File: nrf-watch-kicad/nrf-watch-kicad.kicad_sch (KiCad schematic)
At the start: 78 parts, among them IC1 TLV840MAPL36DBVRQ1, IC2 XC9265C181MR-G, IC3 TPS61023DRLT, IC4 MAX30101EFD+T, M1 Vibrator DC Motor, Q1 DMP2045U-7, Q2 SS8050-G, U1 MAX1811ESA+, U2 DMC2400UV-7, U3 LIS2DS12TR, U4 MX25R6435FZNIL0, U5 u-blox ANNA-B402, U6 DRV2603RUNT, U7 XC9265A331MR-G, U8 TXB0104QRUTRQ1, U9 GC9A01

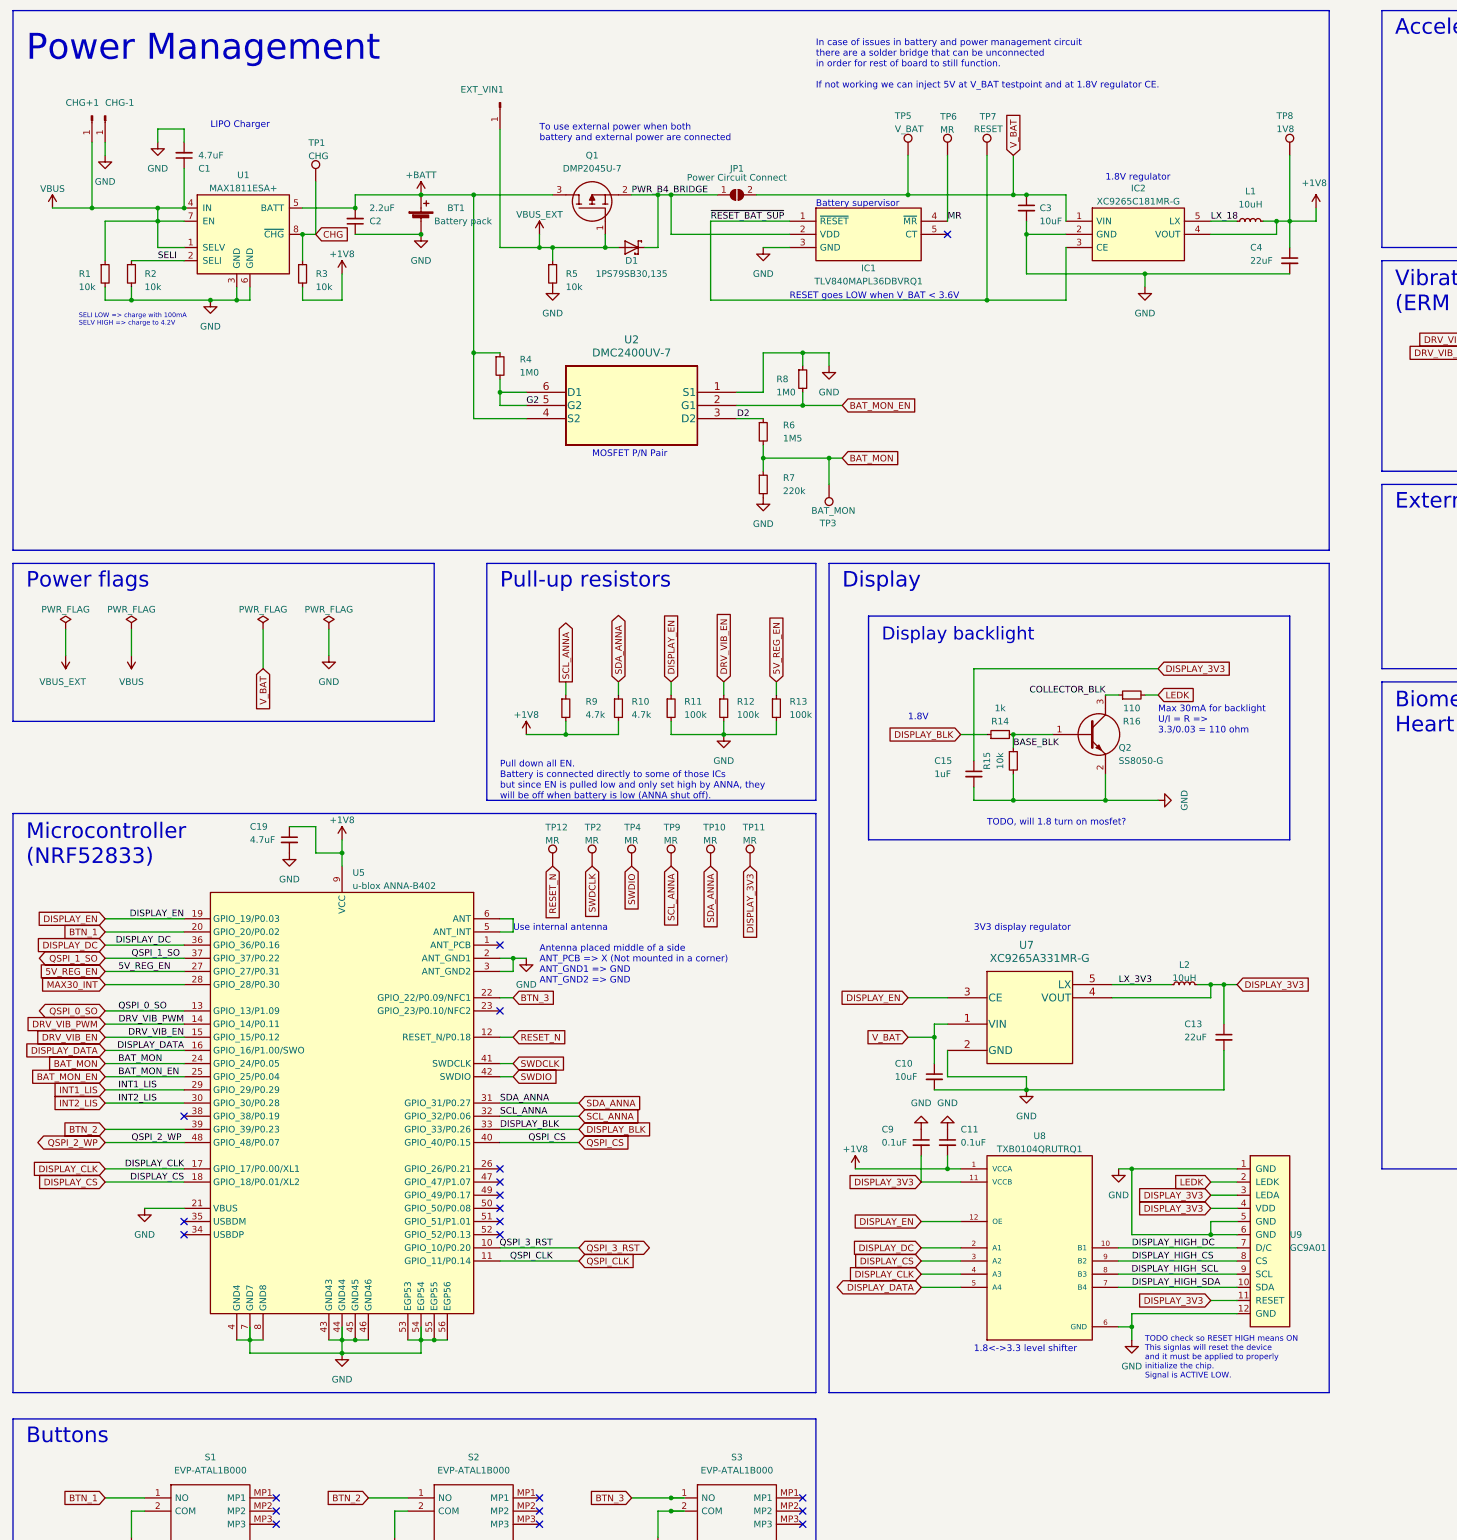
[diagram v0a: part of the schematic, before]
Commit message: Before moving bottom to top
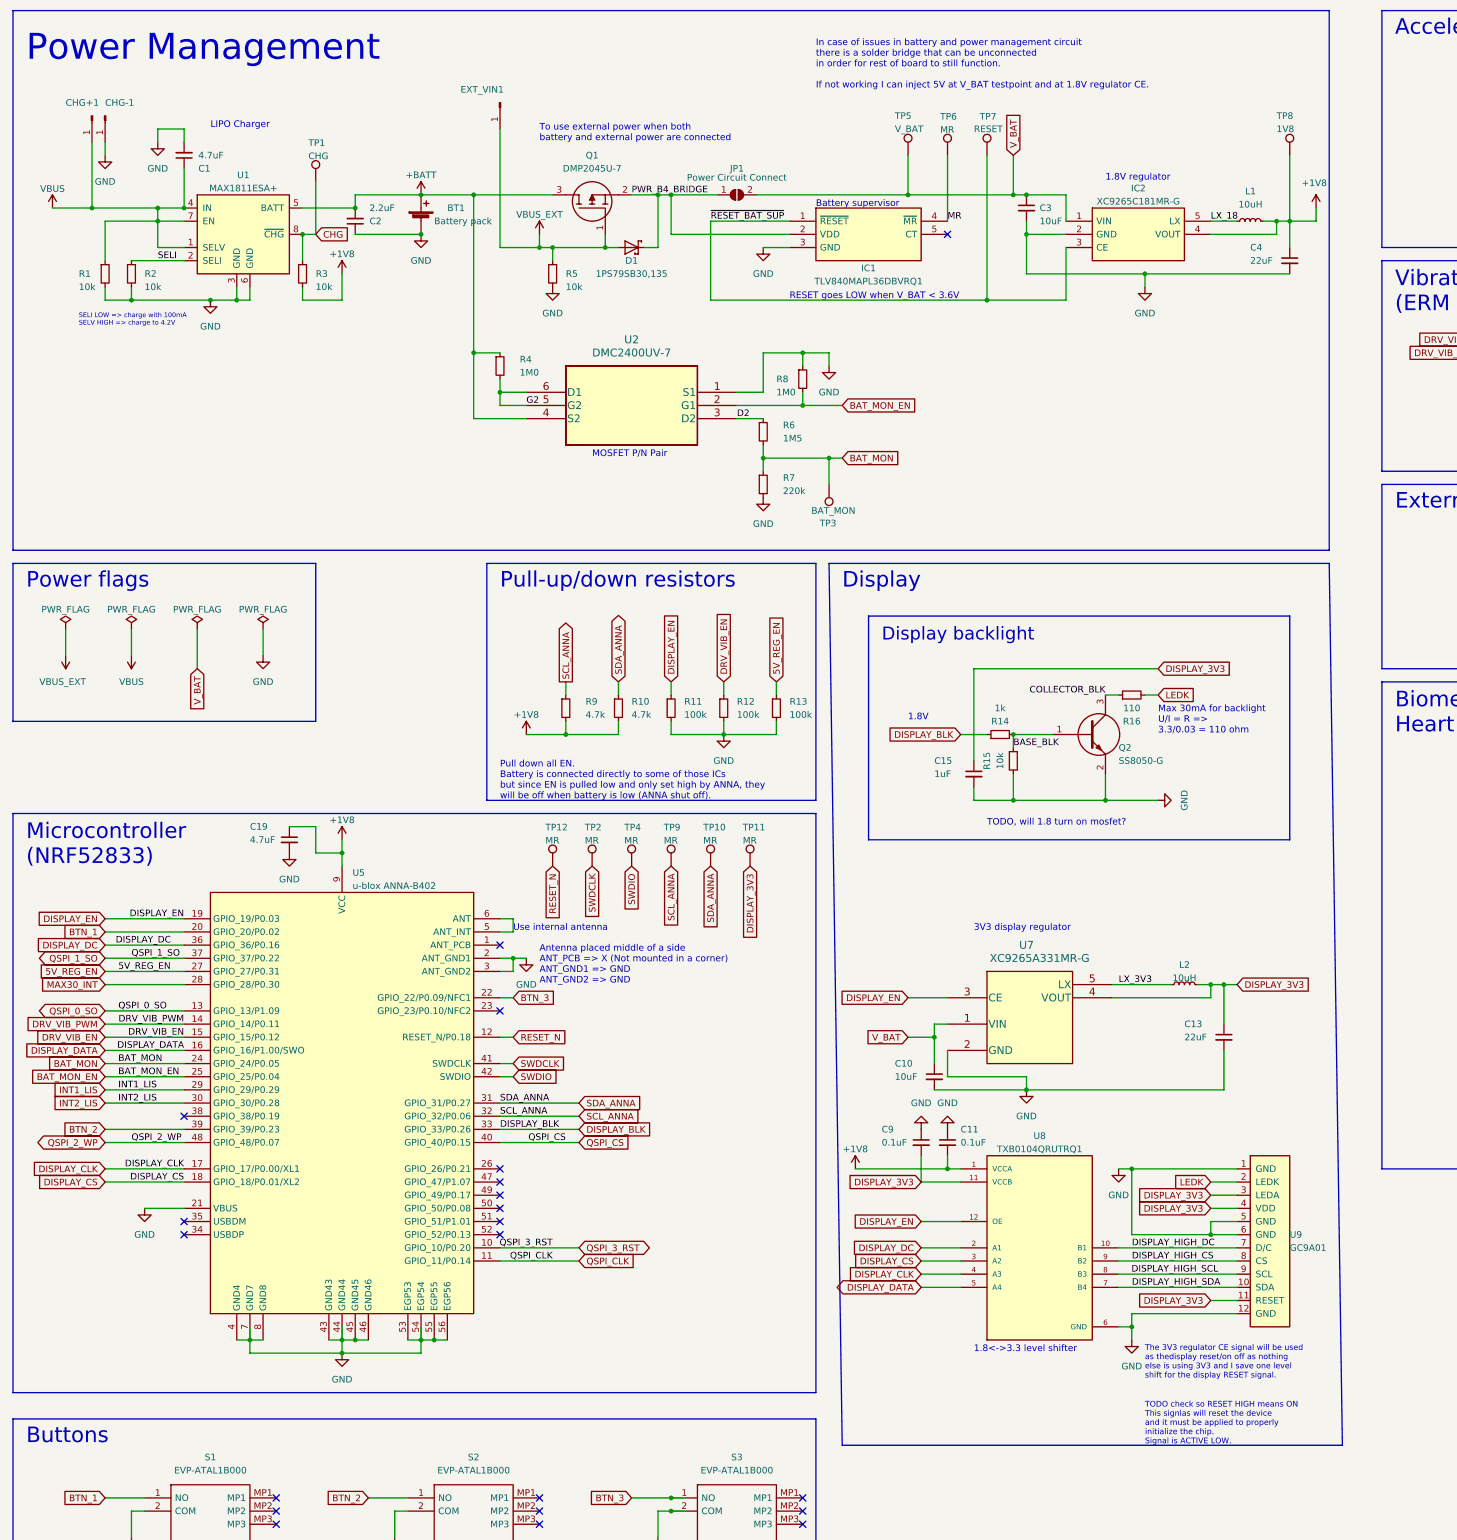
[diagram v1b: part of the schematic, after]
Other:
- note added: "In case of issues in battery and power management circuit there is a solder bridge that can be unconnected in order for rest of board to still function. If not working I can inject 5V at V_BAT testpoint and at 1.8V regulator CE."
- note added: "Pull-up/down resistors"
- note added: "The 3V3 regulator CE signal will be used as thedisplay reset/on off as nothing else is using 3V3 and I save one level shift for the display RESET signal."
- note removed: "In case of issues in battery and power management circuit there are a solder bridge that can be unconnected in order for rest of board to still function. If not working we can inject 5V at V_BAT testpoint and at 1.8V regulator CE."
- note removed: "Pull-up resistors"
- company: Jakob Krantz -> (none)
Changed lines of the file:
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@@
 (kicad_sch (version 20211123) (generator eeschema)
-  (paper "A2")
+  (paper "User" 419.989 340.004)
   (title_block
     (title "Smart Watch")
     (date "2022-09-05")
     (rev "0.1")
-    (company "Jakob Krantz")
   )
   (junction (at 261.62 55.88) (diameter 0) (color 0 0 0 0)
@@
     (stroke (width 0) (type default) (color 0 0 0 0))
   )
-  (polyline (pts (xy 96.52 152.4) (xy 15.24 152.4))
+  (polyline (pts (xy 73.66 152.4) (xy 15.24 152.4))
     (stroke (width 0) (type default) (color 0 0 0 0))
   )
@@
     (stroke (width 0) (type default) (color 0 0 0 0))
   )
-  (polyline (pts (xy 269.24 281.94) (xy 269.24 121.92))
+  (polyline (pts (xy 271.78 292.1) (xy 269.24 121.92))
     (stroke (width 0) (type default) (color 0 0 0 0))
   )
@@
     (stroke (width 0) (type default) (color 0 0 0 0))
   )
-  (polyline (pts (xy 96.52 121.92) (xy 96.52 152.4))
+  (polyline (pts (xy 73.66 121.92) (xy 73.66 152.4))
     (stroke (width 0) (type default) (color 0 0 0 0))
   )
@@
     (stroke (width 0) (type default) (color 0 0 0 0))
   )
-  (wire (pts (xy 63.5 134.62) (xy 63.5 142.24))
+  (wire (pts (xy 50.8 134.62) (xy 50.8 142.24))
     (stroke (width 0) (type default) (color 0 0 0 0))
   )
@@
     (stroke (width 0) (type default) (color 0 0 0 0))
   )
-  (polyline (pts (xy 172.72 121.92) (xy 172.72 281.94))
+  (polyline (pts (xy 172.72 121.92) (xy 175.26 292.1))
     (stroke (width 0) (type default) (color 0 0 0 0))
   )
@@
     (stroke (width 0) (type default) (color 0 0 0 0))
   )
-  (polyline (pts (xy 172.72 281.94) (xy 269.24 281.94))
+  (polyline (pts (xy 175.26 292.1) (xy 271.78 292.1))
     (stroke (width 0) (type default) (color 0 0 0 0))
   )
@@
     (stroke (width 0) (type default) (color 0 0 0 0))
   )
-  (wire (pts (xy 76.2 134.62) (xy 76.2 139.7))
+  (wire (pts (xy 63.5 134.62) (xy 63.5 139.7))
     (stroke (width 0) (type default) (color 0 0 0 0))
   )
@@
     (stroke (width 0) (type default) (color 0 0 0 0))
   )
-  (polyline (pts (xy 15.24 121.92) (xy 96.52 121.92))
+  (polyline (pts (xy 15.24 121.92) (xy 73.66 121.92))
     (stroke (width 0) (type default) (color 0 0 0 0))
   )
@@
     (effects (font (size 1.27 1.27)) (justify left bottom))
   )
-  (text "Pull-up resistors" (at 109.22 127 0)
+  (text "Pull-up/down resistors" (at 109.22 127 0)
     (effects (font (size 3 3)) (justify left bottom))
   )
@@
     (effects (font (size 1.27 1.27)) (justify left bottom))
   )
-  (text "In case of issues in battery and power management circuit \nthere are a solder bridge that can be unconnected\nin order for rest of board to still function.\n\nIf not working we can inject 5V at V_BAT testpoint and at 1.8V regulator CE."
+  (text "In case of issues in battery and power management circuit \nthere is a solder bridge that can be unconnected\nin order for rest of board to still function.\n\nIf not working I can inject 5V at V_BAT testpoint and at 1.8V regulator CE."
     (at 170.18 30.48 0)
     (effects (font (size 1.27 1.27)) (justify left bottom))
@@
     (effects (font (size 1.27 1.27)) (justify left bottom))
   )
+  (text "The 3V3 regulator CE signal will be used\nas thedisplay reset/on off as nothing\nelse is using 3V3 and I save one level\nshift for the display RESET signal."
+    (at 233.68 279.4 0)
+    (effects (font (size 1.1 1.1)) (justify left bottom))
+  )
   (text "Vibration motor\n(ERM Mode)" (at 281.94 73.66 0)
     (effects (font (size 3 3)) (justify left bottom))
   )
   (text "TODO check so RESET HIGH means ON\nThis signlas will reset the device\nand it must be applied to properly\ninitialize the chip.\nSignal is ACTIVE LOW."
-    (at 233.68 279.4 0)
+    (at 233.68 292.1 0)
     (effects (font (size 1.1 1.1)) (justify left bottom))
   )
@@
     )
   )
-  (global_label "V_BAT" (shape input) (at 63.5 142.24 270) (fields_autoplaced)
+  (global_label "V_BAT" (shape input) (at 50.8 142.24 270) (fields_autoplaced)
     (effects (font (size 1.27 1.27)) (justify right))
-    (property "Intersheet References" "${INTERSHEET_REFS}" (id 0) (at 63.5794 150.0355 90)
+    (property "Intersheet References" "${INTERSHEET_REFS}" (id 0) (at 50.8794 150.0355 90)
       (effects (font (size 1.27 1.27)) (justify right) hide)
     )
@@
     (pin "1")
   )
-  (symbol (lib_id "power:GND") (at 76.2 139.7 0) (unit 1)
+  (symbol (lib_id "power:GND") (at 63.5 139.7 0) (unit 1)
     (in_bom yes) (on_board yes)
-    (property "Reference" "#PWR024" (id 0) (at 76.2 146.05 0)
+    (property "Reference" "#PWR024" (id 0) (at 63.5 146.05 0)
       (effects (font (size 1.27 1.27)) hide)
     )
-    (property "Value" "GND" (id 1) (at 76.2 144.78 0))
-    (property "Footprint" "" (id 2) (at 76.2 139.7 0)
+    (property "Value" "GND" (id 1) (at 63.5 144.78 0))
+    (property "Footprint" "" (id 2) (at 63.5 139.7 0)
       (effects (font (size 1.27 1.27)) hide)
     )
-    (property "Datasheet" "" (id 3) (at 76.2 139.7 0)
+    (property "Datasheet" "" (id 3) (at 63.5 139.7 0)
       (effects (font (size 1.27 1.27)) hide)
     )
@@
     (pin "2")
   )
-  (symbol (lib_id "power:PWR_FLAG") (at 76.2 134.62 0) (unit 1)
+  (symbol (lib_id "power:PWR_FLAG") (at 63.5 134.62 0) (unit 1)
     (in_bom yes) (on_board yes) (fields_autoplaced)
-    (property "Reference" "#FLG05" (id 0) (at 76.2 132.715 0)
+    (property "Reference" "#FLG05" (id 0) (at 63.5 132.715 0)
       (effects (font (size 1.27 1.27)) hide)
     )
-    (property "Value" "PWR_FLAG" (id 1) (at 76.2 130.81 0))
-    (property "Footprint" "" (id 2) (at 76.2 134.62 0)
+    (property "Value" "PWR_FLAG" (id 1) (at 63.5 130.81 0))
+    (property "Footprint" "" (id 2) (at 63.5 134.62 0)
       (effects (font (size 1.27 1.27)) hide)
     )
-    (property "Datasheet" "~" (id 3) (at 76.2 134.62 0)
+    (property "Datasheet" "~" (id 3) (at 63.5 134.62 0)
       (effects (font (size 1.27 1.27)) hide)
     )
@@
     (pin "9")
   )
-  (symbol (lib_id "power:PWR_FLAG") (at 63.5 134.62 0) (unit 1)
+  (symbol (lib_id "power:PWR_FLAG") (at 50.8 134.62 0) (unit 1)
     (in_bom yes) (on_board yes) (fields_autoplaced)
-    (property "Reference" "#FLG04" (id 0) (at 63.5 132.715 0)
+    (property "Reference" "#FLG04" (id 0) (at 50.8 132.715 0)
       (effects (font (size 1.27 1.27)) hide)
     )
-    (property "Value" "PWR_FLAG" (id 1) (at 63.5 130.81 0))
-    (property "Footprint" "" (id 2) (at 63.5 134.62 0)
+    (property "Value" "PWR_FLAG" (id 1) (at 50.8 130.81 0))
+    (property "Footprint" "" (id 2) (at 50.8 134.62 0)
       (effects (font (size 1.27 1.27)) hide)
     )
-    (property "Datasheet" "~" (id 3) (at 63.5 134.62 0)
+    (property "Datasheet" "~" (id 3) (at 50.8 134.62 0)
       (effects (font (size 1.27 1.27)) hide)
     )
